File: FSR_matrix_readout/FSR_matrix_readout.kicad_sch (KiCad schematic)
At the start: 7 parts, among them U1 NCD98010XMXTAG, U17 74VHC393FT, U2 NCD98010XMXTAG, U3 TLV9064, U4 TPW4051-QF4R, U5 TPW4051-QF4R

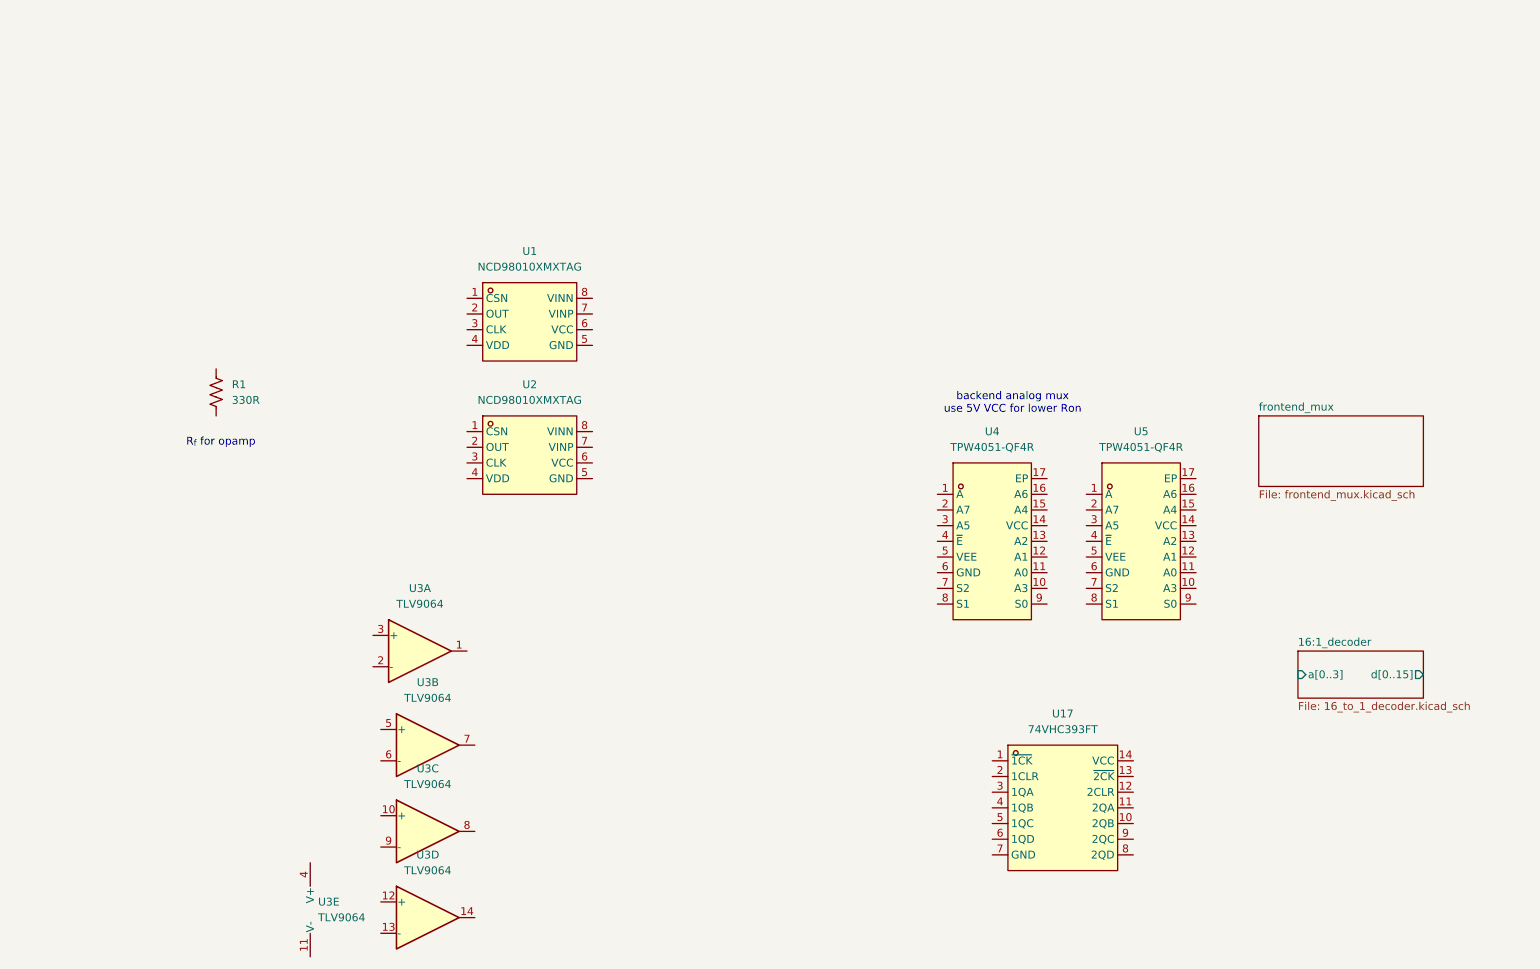
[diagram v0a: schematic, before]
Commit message: done sense opamp module
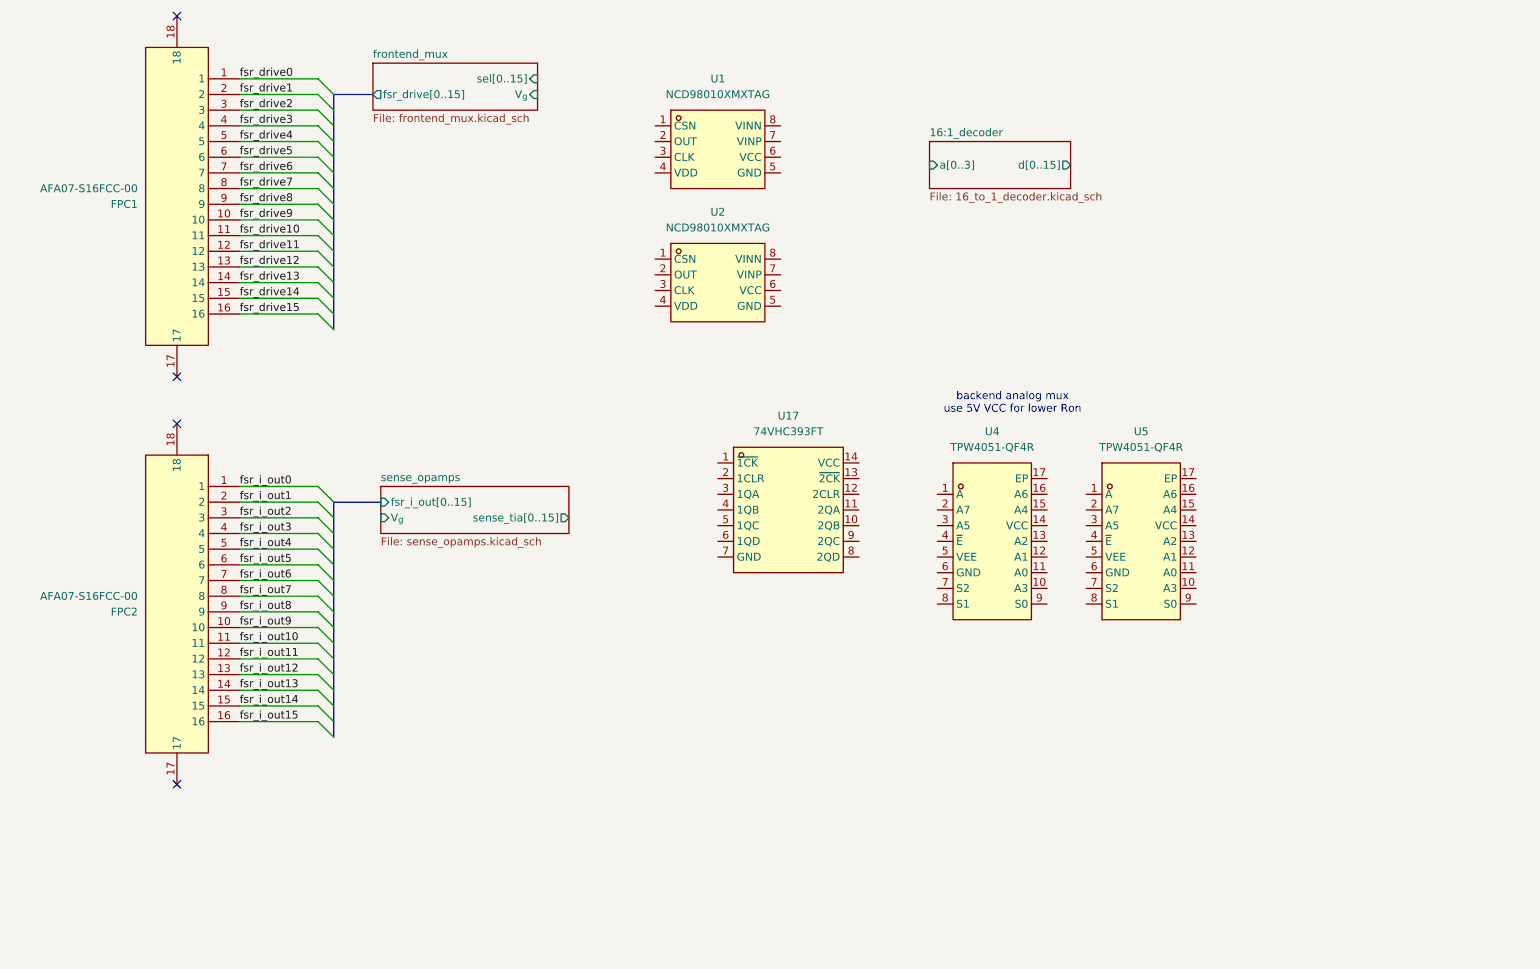
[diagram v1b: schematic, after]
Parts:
- removed R1: 330R, symbol Device:R_US
- removed U3: TLV9064, symbol Amplifier_Operational:TLV9064
- added FPC1, FPC2: AFA07-S16FCC-00, easyeda2kicad:FPC-SMD_16P-P1.00_AFA07-S16FCC-00, symbol lcsc:AFA07-S16FCC-00
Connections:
- new net fsr_drive0: FPC1.1
- new net fsr_drive1: FPC1.2
- new net fsr_drive10: FPC1.11
- new net fsr_drive11: FPC1.12
- new net fsr_drive12: FPC1.13
- new net fsr_drive13: FPC1.14
- new net fsr_drive14: FPC1.15
- new net fsr_drive15: FPC1.16
- new net fsr_drive2: FPC1.3
- new net fsr_drive3: FPC1.4
- new net fsr_drive4: FPC1.5
- new net fsr_drive5: FPC1.6
- new net fsr_drive6: FPC1.7
- new net fsr_drive7: FPC1.8
- new net fsr_drive8: FPC1.9
- new net fsr_drive9: FPC1.10
- new net fsr_i_out0: FPC2.1
- new net fsr_i_out1: FPC2.2
- new net fsr_i_out10: FPC2.11
- new net fsr_i_out11: FPC2.12
- new net fsr_i_out12: FPC2.13
- new net fsr_i_out13: FPC2.14
- new net fsr_i_out14: FPC2.15
- new net fsr_i_out15: FPC2.16
- new net fsr_i_out2: FPC2.3
- new net fsr_i_out3: FPC2.4
- new net fsr_i_out4: FPC2.5
- new net fsr_i_out5: FPC2.6
- new net fsr_i_out6: FPC2.7
- new net fsr_i_out7: FPC2.8
- new net fsr_i_out8: FPC2.9
- new net fsr_i_out9: FPC2.10
- no-connect marks 0 -> 4
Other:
- added sheet sense_opamps (sense_opamps.kicad_sch)
- sheet frontend_mux ports: added V_{g}, fsr_drive[0..15], sel[0..15]; removed none
- note removed: "R_{f} for opamp"
- moved on the sheet: U1, U17, U2
